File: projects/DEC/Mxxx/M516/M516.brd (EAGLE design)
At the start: 125.7 x 62.2 mm, 45 parts

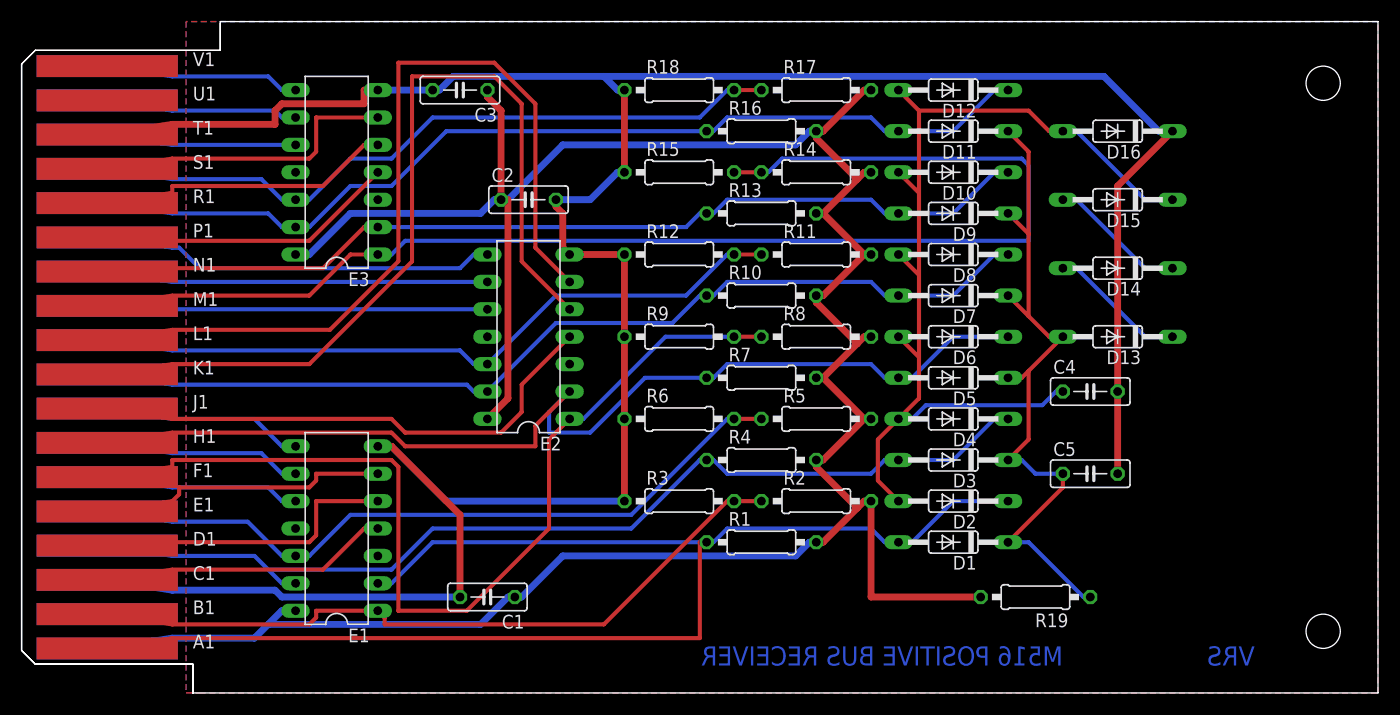
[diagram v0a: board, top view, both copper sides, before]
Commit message: Walk the project tree, making things pass current design rules.
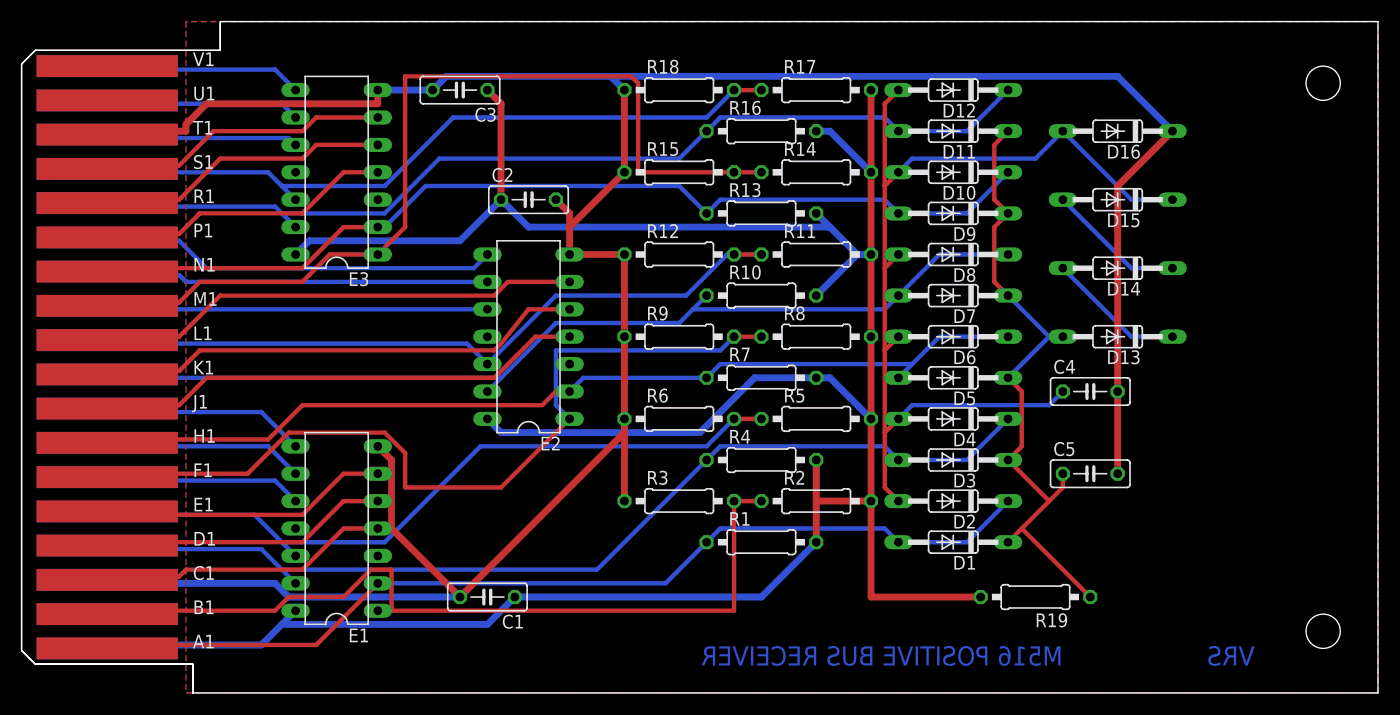
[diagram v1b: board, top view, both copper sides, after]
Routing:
- net A1: track 127.2 -> 90.2 mm
- net M1: track 122.7 -> 86.2 mm
- net K1: track 81.5 -> 45.6 mm
- net L1: track 80.2 -> 45.1 mm
- net VCC: track 245.8 -> 263.3 mm
- net F1: track 90.3 -> 77.6 mm
- net B1: track 67.2 -> 77.6 mm
- net H1: track 98.6 -> 89.4 mm
- net +3.2V: track 66.8 -> 60.9 mm
- net GND: track 265.0 -> 260.2 mm
- net J1: track 48.6 -> 45.6 mm
- net N1: track 88.2 -> 90.5 mm
- net K2: track 90.2 -> 92.0 mm
- net D1: track 28.5 -> 26.8 mm
- net S1: track 28.6 -> 27.1 mm
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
